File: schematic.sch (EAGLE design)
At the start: 15 parts, among them IC1 ESP-WROOM-02, IC2 SN54HC595, IC3 TD62083APG

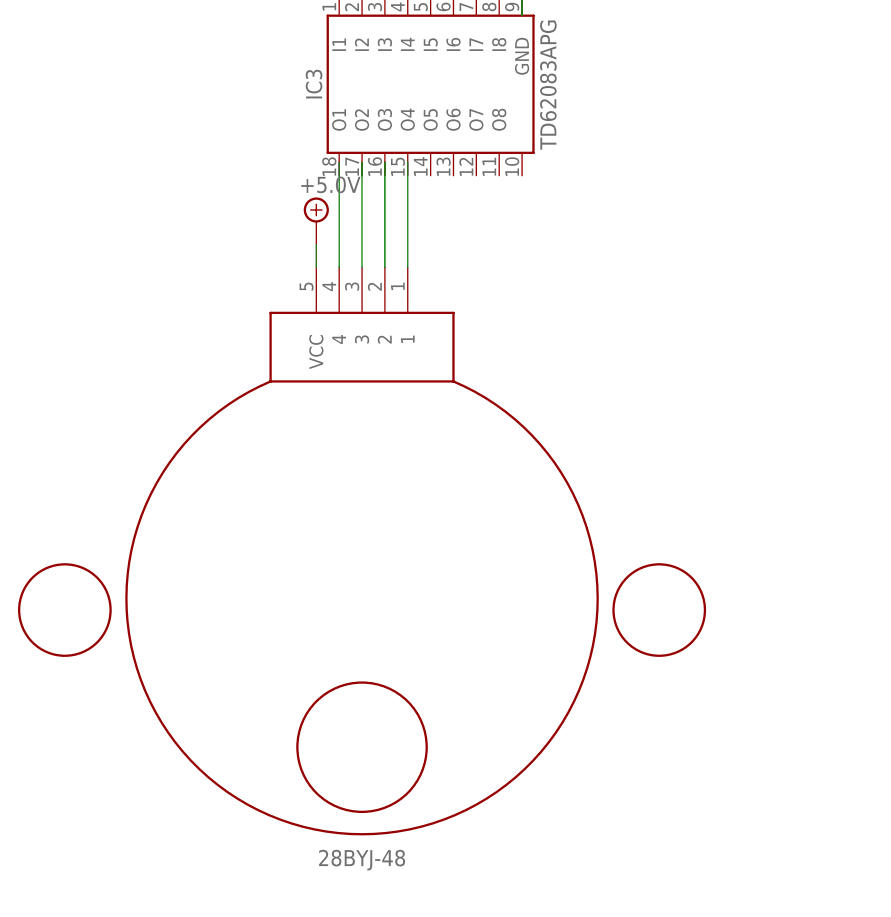
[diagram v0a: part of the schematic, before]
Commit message: fix sche.
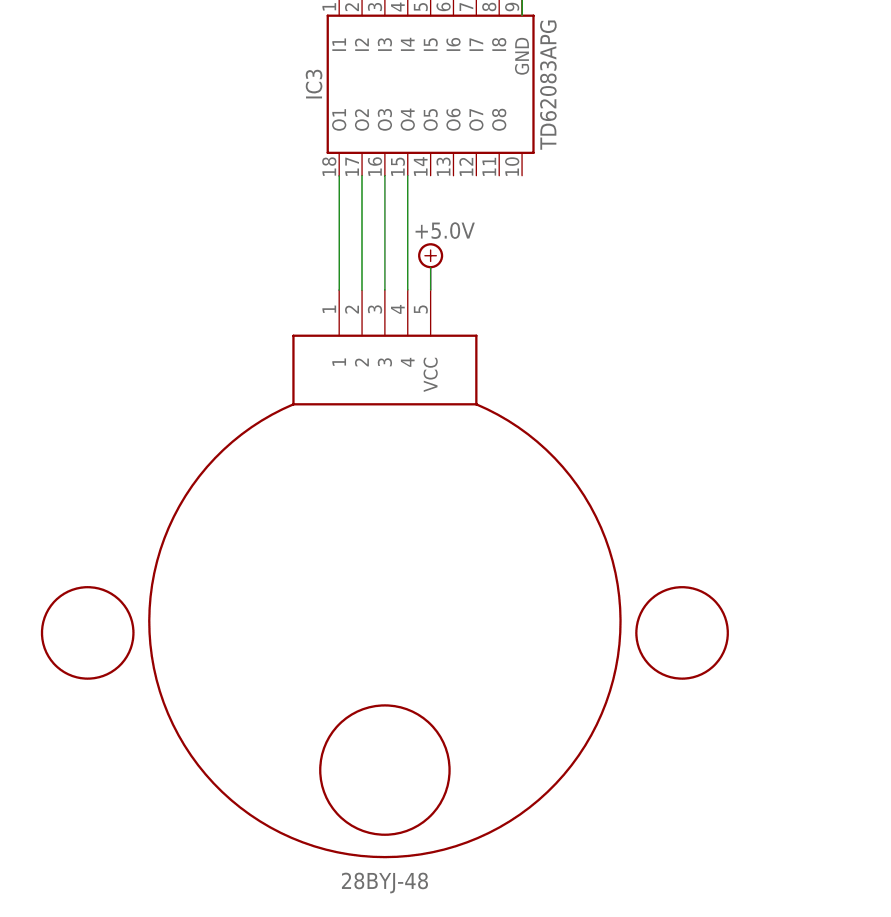
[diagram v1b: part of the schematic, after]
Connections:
- new net N$9: IC3.O1, U$1.1
- net +3.3V: no longer U$1.VCC
- net N$11: now also IC3.O2, U$1.2; no longer IC3.O1, U$1.4
- net N$12: now also IC3.O3; no longer IC3.O2
- net N$13: now also IC3.O4, U$1.4; no longer IC3.O3, U$1.2
- net N$14: now also U$1.VCC; no longer IC3.O4, U$1.1
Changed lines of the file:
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@@
 <instance part="SUPPLY15" gate="P" x="114.3" y="139.7"/>
 <instance part="IC2" gate="G$1" x="99.06" y="127"/>
-<instance part="U$1" gate="G$1" x="53.34" y="43.18" rot="R180"/>
+<instance part="U$1" gate="G$1" x="55.88" y="40.64" rot="MR180"/>
 <instance part="U$2" gate="G$1" x="218.44" y="43.18" rot="R180"/>
 <instance part="R8" gate="G$1" x="218.44" y="137.16" rot="R90"/>
@@
 <instance part="R6" gate="G$1" x="218.44" y="116.84" rot="R90"/>
 <instance part="SUPPLY5" gate="GND" x="218.44" y="144.78" rot="R180"/>
-<instance part="SUPPLY12" gate="P" x="48.26" y="86.36"/>
+<instance part="SUPPLY12" gate="P" x="60.96" y="81.28"/>
 <instance part="SUPPLY13" gate="GND" x="213.36" y="60.96" rot="R180"/>
 <instance part="SUPPLY14" gate="P" x="223.52" y="60.96"/>
@@
 <pinref part="SUPPLY15" gate="P" pin="+3.3V"/>
 <wire x1="114.3" y1="134.62" x2="114.3" y2="137.16" width="0.1524" layer="91"/>
-</segment>
-<segment>
-<pinref part="U$1" gate="G$1" pin="VCC"/>
-<pinref part="SUPPLY12" gate="P" pin="+3.3V"/>
-<wire x1="48.26" y1="81.28" x2="48.26" y2="83.82" width="0.1524" layer="91"/>
 </segment>
 <segment>
@@
 </segment>
 </net>
-<net name="N$11" class="0">
-<segment>
-<pinref part="IC3" gate="G$1" pin="O1"/>
-<pinref part="U$1" gate="G$1" pin="4"/>
-<wire x1="50.8" y1="81.28" x2="50.8" y2="92.964" width="0.1524" layer="91"/>
-</segment>
-</net>
-<net name="N$12" class="0">
-<segment>
-<pinref part="IC3" gate="G$1" pin="O2"/>
-<pinref part="U$1" gate="G$1" pin="3"/>
-<wire x1="53.34" y1="81.28" x2="53.34" y2="92.964" width="0.1524" layer="91"/>
-</segment>
-</net>
-<net name="N$13" class="0">
-<segment>
-<pinref part="IC3" gate="G$1" pin="O3"/>
-<pinref part="U$1" gate="G$1" pin="2"/>
-<wire x1="55.88" y1="81.28" x2="55.88" y2="92.964" width="0.1524" layer="91"/>
-</segment>
-</net>
-<net name="N$14" class="0">
-<segment>
-<pinref part="IC3" gate="G$1" pin="O4"/>
-<pinref part="U$1" gate="G$1" pin="1"/>
-<wire x1="58.42" y1="81.28" x2="58.42" y2="92.964" width="0.1524" layer="91"/>
-</segment>
-</net>
 <net name="N$2" class="0">
 <segment>
@@
 </segment>
 </net>
+<net name="N$9" class="0">
+<segment>
+<pinref part="U$1" gate="G$1" pin="1"/>
+<pinref part="IC3" gate="G$1" pin="O1"/>
+<wire x1="50.8" y1="78.74" x2="50.8" y2="91.44" width="0.1524" layer="91"/>
+</segment>
+</net>
+<net name="N$11" class="0">
+<segment>
+<pinref part="U$1" gate="G$1" pin="2"/>
+<pinref part="IC3" gate="G$1" pin="O2"/>
+<wire x1="53.34" y1="78.74" x2="53.34" y2="91.44" width="0.1524" layer="91"/>
+</segment>
+</net>
+<net name="N$12" class="0">
+<segment>
+<pinref part="U$1" gate="G$1" pin="3"/>
+<pinref part="IC3" gate="G$1" pin="O3"/>
+<wire x1="55.88" y1="78.74" x2="55.88" y2="91.44" width="0.1524" layer="91"/>
+</segment>
+</net>
+<net name="N$13" class="0">
+<segment>
+<pinref part="U$1" gate="G$1" pin="4"/>
+<pinref part="IC3" gate="G$1" pin="O4"/>
+<wire x1="58.42" y1="78.74" x2="58.42" y2="91.44" width="0.1524" layer="91"/>
+</segment>
+</net>
+<net name="N$14" class="0">
+<segment>
+<pinref part="U$1" gate="G$1" pin="VCC"/>
+<wire x1="60.96" y1="78.74" x2="60.96" y2="81.28" width="0.1524" layer="91"/>
+</segment>
+</net>
